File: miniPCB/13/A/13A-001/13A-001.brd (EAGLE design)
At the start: 12 parts

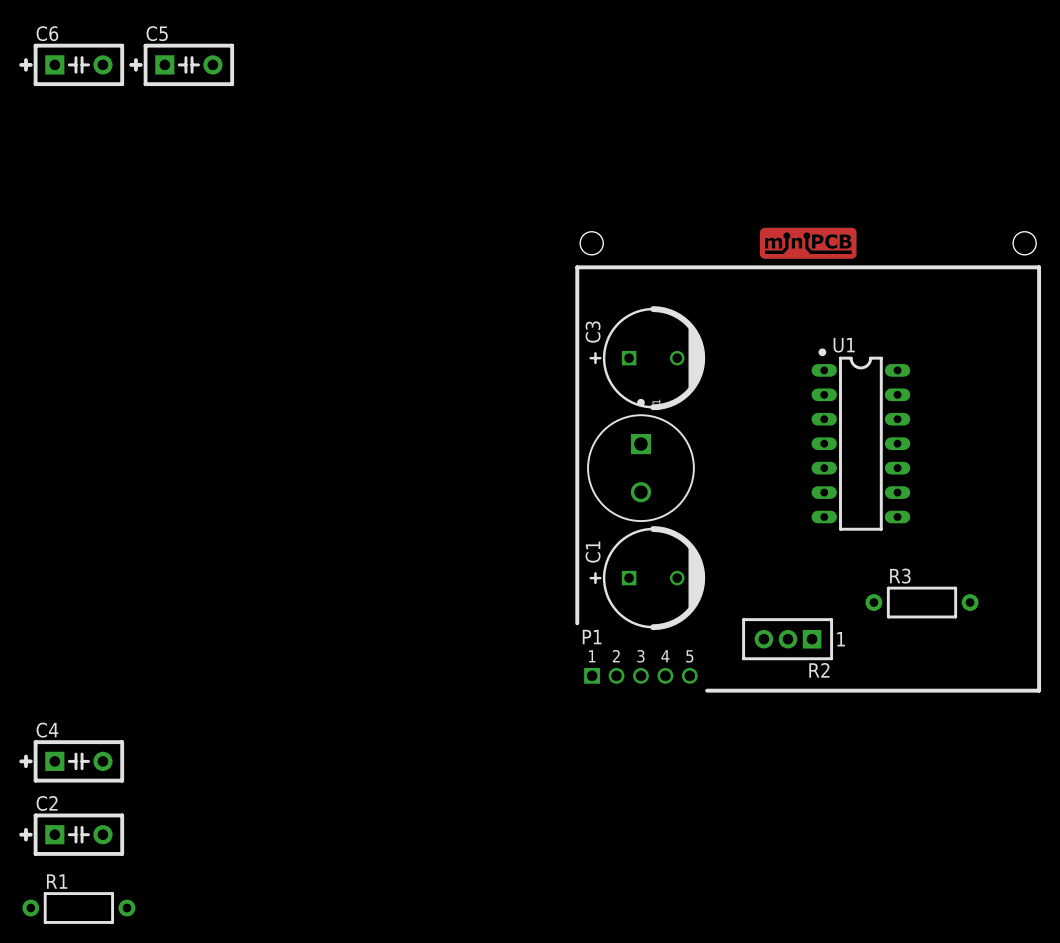
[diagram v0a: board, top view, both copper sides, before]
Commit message: NM.03SEP2023
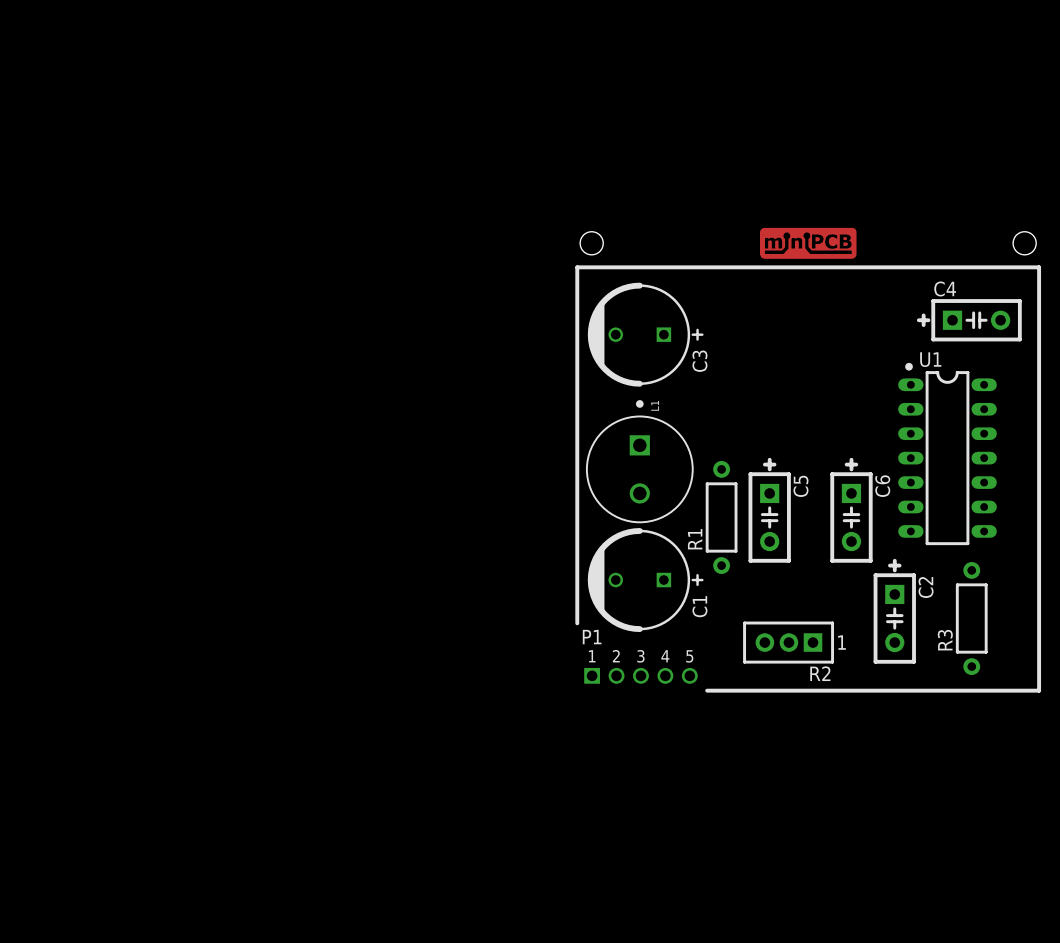
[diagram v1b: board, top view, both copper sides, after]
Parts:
- moved C4 104.0 mm to (42.5, 39.5)
- moved C6 93.1 mm to (29.5, 19.0), turned to 270 degrees
- moved C2 87.7 mm to (34.0, 8.50), turned to 270 degrees
- moved R1 78.2 mm to (16.0, 19.0), turned to 90 degrees
- moved C5 76.5 mm to (21.0, 19.0), turned to 270 degrees
- moved U1 9.12 mm to (39.5, 25.2)
- moved R3 5.43 mm to (42.0, 8.50), turned to 90 degrees
- moved C3 2.81 mm to (7.50, 38.0), turned to 180 degrees
- moved C1 1.40 mm to (7.50, 12.5), turned to 180 degrees
- moved R2 0.36 mm to (25.5, 6.00)
- moved L1 0.18 mm to (7.50, 24.0)
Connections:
- removed net N$10: P1-.2
- net GND: now also P1-.1
- net N$5: now also P1-.2; no longer P1-.1
